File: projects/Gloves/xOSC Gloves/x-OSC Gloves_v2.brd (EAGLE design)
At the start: 102.5 x 92.7 mm, 58 parts

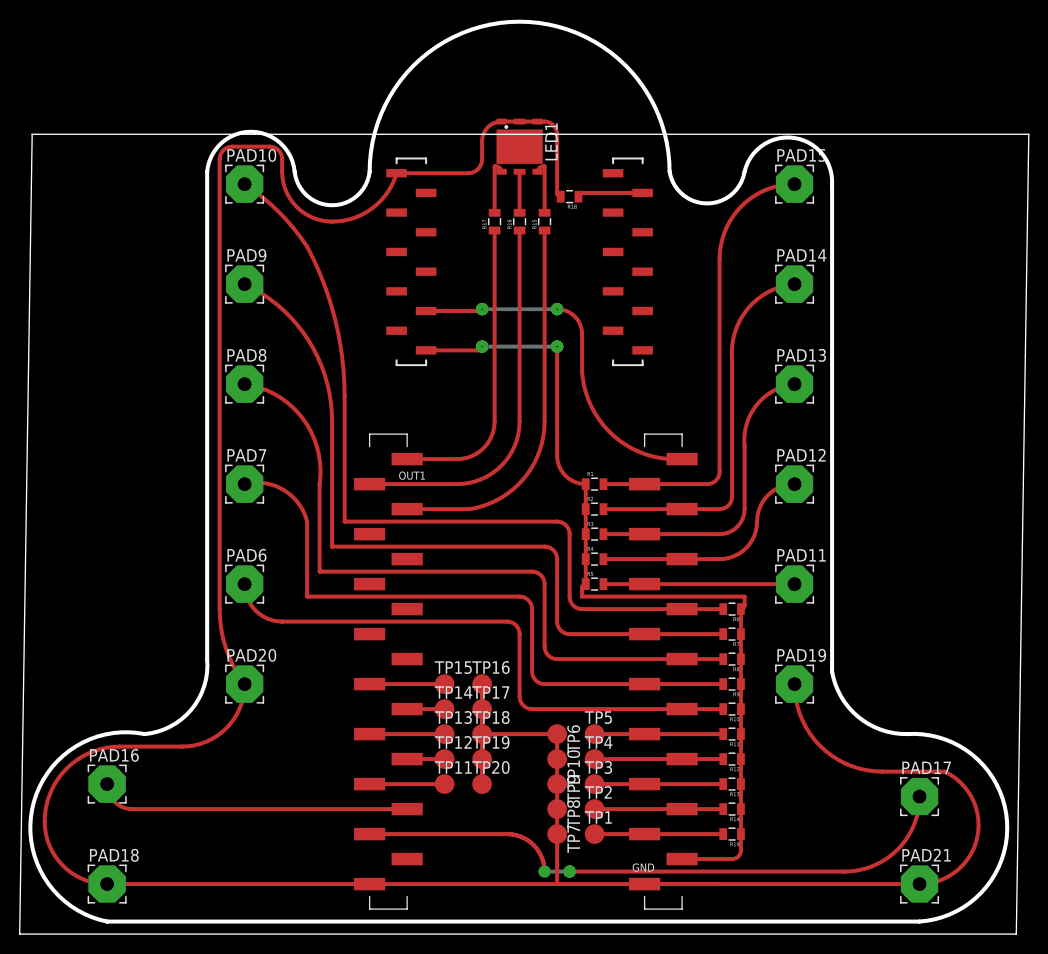
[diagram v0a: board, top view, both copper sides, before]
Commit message: MegaGlove final baord
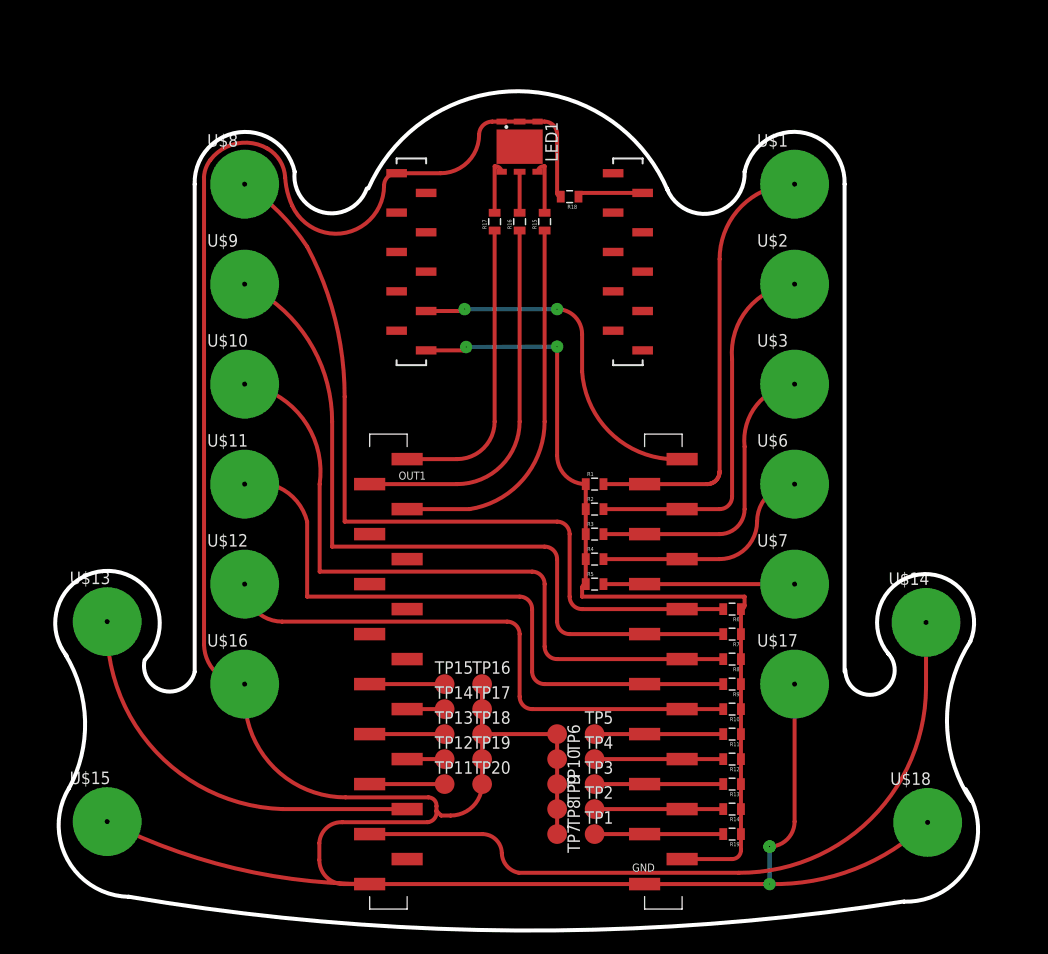
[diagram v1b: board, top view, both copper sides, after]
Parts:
- removed PAD10, PAD11, PAD12, PAD13, PAD14, PAD15, PAD16, PAD17, PAD18, PAD19, PAD20, PAD21, PAD6, PAD7, PAD8, PAD9: (no value), wirepad:3,81/1,4
- added U$1, U$10, U$11, U$12, U$13, U$14, U$15, U$16, U$17, U$18, U$2, U$3, U$6, U$7, U$8, U$9: SNAP-PAD_7MM_ROUND, hannahsEagleLib:SNAP-PAD_7MM_RD
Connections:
- net GND: now also U$15.P$1, U$16.P$1, U$17.P$1, U$18.P$1; no longer PAD18.1, PAD19.1, PAD20.1, PAD21.1
- net N$12: now also U$8.P$1; no longer PAD10.1
- net N$13: now also U$9.P$1; no longer PAD9.1
- net N$14: now also U$10.P$1; no longer PAD8.1
- net N$15: now also U$11.P$1; no longer PAD7.1
- net N$16: now also U$12.P$1; no longer PAD6.1
- net N$23: now also U$13.P$1; no longer PAD16.1
- net N$24: now also U$14.P$1; no longer PAD17.1
- net N$4: now also U$1.P$1; no longer PAD15.1
- net N$6: now also U$2.P$1; no longer PAD14.1
- net N$7: now also U$3.P$1; no longer PAD13.1
- net N$8: now also U$6.P$1; no longer PAD12.1
- net N$9: now also U$7.P$1; no longer PAD11.1
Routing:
- net N$23: track 31.5 -> 38.8 mm
- net N$24: track 66.0 -> 72.6 mm, vias 2 -> 0
- net N$4: track 44.7 -> 46.5 mm
- net GND: track 298.4 -> 297.2 mm, vias 0 -> 1
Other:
- board size 102.5 x 92.7 mm -> 93.8 x 85.3 mm
